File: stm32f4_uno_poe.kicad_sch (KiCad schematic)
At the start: 12 parts, among them J101 STM32 GPIO, J102 Digital/PWM, J103 STM32 GPIO, J104 STM32 GPIO, J105 STM32 GPIO, J106 Power, J107 Conn_01x04, J108 Ethernet, J109 STM32 GPIO, J110 Digital/PWM, J111 Analog, J112 Barrel_Jack

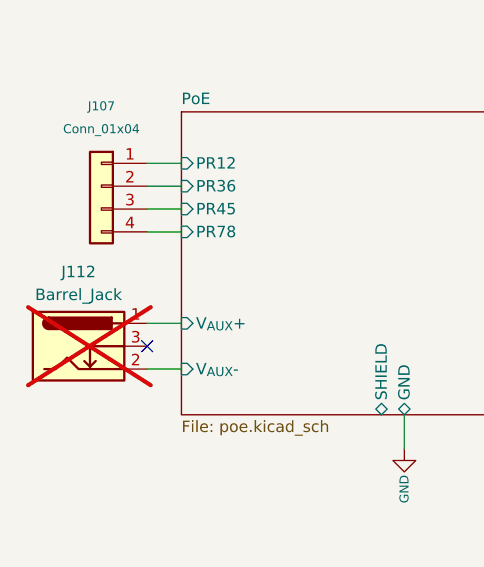
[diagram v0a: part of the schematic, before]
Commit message: WIP
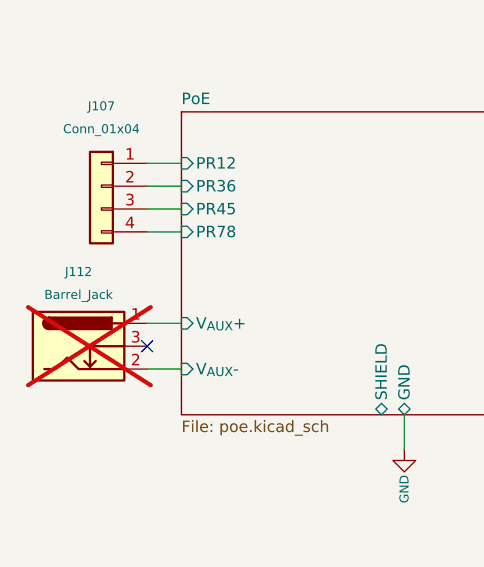
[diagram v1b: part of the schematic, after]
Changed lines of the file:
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@@
     )
     (property "Description" "" (at 262.255 37.465 0)
-      (effects (font (size 1.27 1.27)) hide)
+      (effects (font (size 1 1)) hide)
     )
     (property "Manufacturer" "" (at 262.255 37.465 0)
-      (effects (font (size 1.27 1.27)) hide)
+      (effects (font (size 1 1)) hide)
     )
     (property "Partnumber" "" (at 262.255 37.465 0)
-      (effects (font (size 1.27 1.27)) hide)
+      (effects (font (size 1 1)) hide)
     )
     (property "JLCPCB Part #" "" (at 262.255 37.465 0)
-      (effects (font (size 1.27 1.27)) hide)
+      (effects (font (size 1 1)) hide)
     )
     (property "isBasicPart" "" (at 262.255 37.465 0)
-      (effects (font (size 1.27 1.27)) hide)
+      (effects (font (size 1 1)) hide)
     )
     (property "Description" "" (at 262.255 37.465 0)
-      (effects (font (size 1.27 1.27)) hide)
+      (effects (font (size 1 1)) hide)
     )
     (property "Manufacturer" "" (at 262.255 37.465 0)
-      (effects (font (size 1.27 1.27)) hide)
+      (effects (font (size 1 1)) hide)
     )
     (property "Partnumber" "" (at 262.255 37.465 0)
-      (effects (font (size 1.27 1.27)) hide)
+      (effects (font (size 1 1)) hide)
     )
     (property "JLCPCB Part #" "" (at 262.255 37.465 0)
-      (effects (font (size 1.27 1.27)) hide)
+      (effects (font (size 1 1)) hide)
     )
     (property "isBasicPart" "" (at 262.255 37.465 0)
-      (effects (font (size 1.27 1.27)) hide)
+      (effects (font (size 1 1)) hide)
     )
     (pin "1")
@@
     )
     (property "Description" "" (at 262.255 67.945 0)
-      (effects (font (size 1.27 1.27)) hide)
+      (effects (font (size 1 1)) hide)
     )
     (property "Manufacturer" "" (at 262.255 67.945 0)
-      (effects (font (size 1.27 1.27)) hide)
+      (effects (font (size 1 1)) hide)
     )
     (property "Partnumber" "" (at 262.255 67.945 0)
-      (effects (font (size 1.27 1.27)) hide)
+      (effects (font (size 1 1)) hide)
     )
     (property "JLCPCB Part #" "" (at 262.255 67.945 0)
-      (effects (font (size 1.27 1.27)) hide)
+      (effects (font (size 1 1)) hide)
     )
     (property "isBasicPart" "" (at 262.255 67.945 0)
-      (effects (font (size 1.27 1.27)) hide)
+      (effects (font (size 1 1)) hide)
     )
     (property "Description" "" (at 262.255 67.945 0)
-      (effects (font (size 1.27 1.27)) hide)
+      (effects (font (size 1 1)) hide)
     )
     (property "Manufacturer" "" (at 262.255 67.945 0)
-      (effects (font (size 1.27 1.27)) hide)
+      (effects (font (size 1 1)) hide)
     )
     (property "Partnumber" "" (at 262.255 67.945 0)
-      (effects (font (size 1.27 1.27)) hide)
+      (effects (font (size 1 1)) hide)
     )
     (property "JLCPCB Part #" "" (at 262.255 67.945 0)
-      (effects (font (size 1.27 1.27)) hide)
+      (effects (font (size 1 1)) hide)
     )
     (property "isBasicPart" "" (at 262.255 67.945 0)
-      (effects (font (size 1.27 1.27)) hide)
+      (effects (font (size 1 1)) hide)
     )
     (pin "1")
@@
     (in_bom yes) (on_board yes) (dnp yes) (fields_autoplaced)
     (property "Reference" "J112" (at 52.07 69.215 0)
-      (effects (font (size 1.27 1.27)))
+      (effects (font (size 1 1)))
     )
     (property "Value" "Barrel_Jack" (at 52.07 71.755 0)
-      (effects (font (size 1.27 1.27)))
+      (effects (font (size 1 1)))
     )
     (property "Footprint" "Connector_BarrelJack:BarrelJack_CUI_PJ-102AH_Horizontal" (at 53.34 78.486 0)
-      (effects (font (size 1.27 1.27)) hide)
+      (effects (font (size 1 1)) hide)
     )
     (property "Datasheet" "~" (at 53.34 78.486 0)
-      (effects (font (size 1.27 1.27)) hide)
+      (effects (font (size 1 1)) hide)
     )
     (property "Description" "" (at 52.07 77.47 0)
-      (effects (font (size 1.27 1.27)) hide)
+      (effects (font (size 1 1)) hide)
     )
     (property "Manufacturer" "CUI Devices" (at 52.07 77.47 0)
-      (effects (font (size 1.27 1.27)) hide)
+      (effects (font (size 1 1)) hide)
     )
     (property "Partnumber" "PJ-102AH" (at 52.07 77.47 0)
-      (effects (font (size 1.27 1.27)) hide)
+      (effects (font (size 1 1)) hide)
     )
     (property "JLCPCB Part #" "" (at 52.07 77.47 0)
-      (effects (font (size 1.27 1.27)) hide)
+      (effects (font (size 1 1)) hide)
     )
     (property "isBasicPart" "NO" (at 52.07 77.47 0)
-      (effects (font (size 1.27 1.27)) hide)
+      (effects (font (size 1 1)) hide)
     )
     (pin "1")
@@
     )
     (property "Description" "" (at 54.61 59.69 0)
-      (effects (font (size 1.27 1.27)) hide)
+      (effects (font (size 1 1)) hide)
     )
     (property "Manufacturer" "" (at 54.61 59.69 0)
-      (effects (font (size 1.27 1.27)) hide)
+      (effects (font (size 1 1)) hide)
     )
     (property "Partnumber" "" (at 54.61 59.69 0)
-      (effects (font (size 1.27 1.27)) hide)
+      (effects (font (size 1 1)) hide)
     )
     (property "JLCPCB Part #" "" (at 54.61 59.69 0)
-      (effects (font (size 1.27 1.27)) hide)
+      (effects (font (size 1 1)) hide)
     )
     (property "isBasicPart" "" (at 54.61 59.69 0)
-      (effects (font (size 1.27 1.27)) hide)
+      (effects (font (size 1 1)) hide)
     )
     (property "Description" "" (at 54.61 59.69 0)
-      (effects (font (size 1.27 1.27)) hide)
+      (effects (font (size 1 1)) hide)
     )
     (property "Manufacturer" "" (at 54.61 59.69 0)
-      (effects (font (size 1.27 1.27)) hide)
+      (effects (font (size 1 1)) hide)
     )
     (property "Partnumber" "" (at 54.61 59.69 0)
-      (effects (font (size 1.27 1.27)) hide)
+      (effects (font (size 1 1)) hide)
     )
     (property "JLCPCB Part #" "" (at 54.61 59.69 0)
-      (effects (font (size 1.27 1.27)) hide)
+      (effects (font (size 1 1)) hide)
     )
     (property "isBasicPart" "" (at 54.61 59.69 0)
-      (effects (font (size 1.27 1.27)) hide)
+      (effects (font (size 1 1)) hide)
     )
     (pin "1")
@@
     )
     (property "Description" "" (at 204.47 42.545 0)
-      (effects (font (size 1.27 1.27)) hide)
+      (effects (font (size 1 1)) hide)
     )
     (property "Manufacturer" "" (at 204.47 42.545 0)
-      (effects (font (size 1.27 1.27)) hide)
+      (effects (font (size 1 1)) hide)
     )
     (property "Partnumber" "" (at 204.47 42.545 0)
-      (effects (font (size 1.27 1.27)) hide)
+      (effects (font (size 1 1)) hide)
     )
     (property "JLCPCB Part #" "" (at 204.47 42.545 0)
-      (effects (font (size 1.27 1.27)) hide)
+      (effects (font (size 1 1)) hide)
     )
     (property "isBasicPart" "" (at 204.47 42.545 0)
-      (effects (font (size 1.27 1.27)) hide)
+      (effects (font (size 1 1)) hide)
     )
     (property "Description" "" (at 204.47 42.545 0)
-      (effects (font (size 1.27 1.27)) hide)
+      (effects (font (size 1 1)) hide)
     )
     (property "Manufacturer" "" (at 204.47 42.545 0)
-      (effects (font (size 1.27 1.27)) hide)
+      (effects (font (size 1 1)) hide)
     )
     (property "Partnumber" "" (at 204.47 42.545 0)
-      (effects (font (size 1.27 1.27)) hide)
+      (effects (font (size 1 1)) hide)
     )
     (property "JLCPCB Part #" "" (at 204.47 42.545 0)
-      (effects (font (size 1.27 1.27)) hide)
+      (effects (font (size 1 1)) hide)
     )
     (property "isBasicPart" "" (at 204.47 42.545 0)
-      (effects (font (size 1.27 1.27)) hide)
+      (effects (font (size 1 1)) hide)
     )
     (pin "1")
@@
     )
     (property "Description" "" (at 204.47 67.945 0)
-      (effects (font (size 1.27 1.27)) hide)
+      (effects (font (size 1 1)) hide)
     )
     (property "Manufacturer" "" (at 204.47 67.945 0)
-      (effects (font (size 1.27 1.27)) hide)
+      (effects (font (size 1 1)) hide)
     )
     (property "Partnumber" "" (at 204.47 67.945 0)
-      (effects (font (size 1.27 1.27)) hide)
+      (effects (font (size 1 1)) hide)
     )
     (property "JLCPCB Part #" "" (at 204.47 67.945 0)
-      (effects (font (size 1.27 1.27)) hide)
+      (effects (font (size 1 1)) hide)
     )
     (property "isBasicPart" "" (at 204.47 67.945 0)
-      (effects (font (size 1.27 1.27)) hide)
+      (effects (font (size 1 1)) hide)
     )
     (property "Description" "" (at 204.47 67.945 0)
-      (effects (font (size 1.27 1.27)) hide)
+      (effects (font (size 1 1)) hide)
     )
     (property "Manufacturer" "" (at 204.47 67.945 0)
-      (effects (font (size 1.27 1.27)) hide)
+      (effects (font (size 1 1)) hide)
     )
     (property "Partnumber" "" (at 204.47 67.945 0)
-      (effects (font (size 1.27 1.27)) hide)
+      (effects (font (size 1 1)) hide)
     )
     (property "JLCPCB Part #" "" (at 204.47 67.945 0)
-      (effects (font (size 1.27 1.27)) hide)
+      (effects (font (size 1 1)) hide)
     )
     (property "isBasicPart" "" (at 204.47 67.945 0)
-      (effects (font (size 1.27 1.27)) hide)
-    )
-    (pin "1")
+      (effects (font (size 1 1)) hide)
+    )
+    (pin "1")
